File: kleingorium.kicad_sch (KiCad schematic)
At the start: 47 parts, among them J1 4017 Pins, J10 VCC, J11 GND, J12 4046 Comp In, J13 Select, J14 Input, J15 4046 SigIn, J16 4046 Comp, J17 Output, J18 4046 Comp In, J19 4046 Out, J2 4040 Output, J20 4040 Input, J21 4040 Output, J22 4017 Pins, J23 VCC, J24 GND, J25 4017 Fdbk, J26 4017 Fdbk, J3 4040 Input, J4 4046 Out, J5 4046 Comp, J6 Select, J7 Output, J8 Input, J9 4046 SigIn, Q1 2N3904, Q2 2N3904, Q3 2N3904, Q4 2N3904, Q5 2N3904, Q6 2N3904, SW1 4017 Feedback, SW2 4046 CompIn, SW3 Chain, SW4 4017 Feedback, SW5 4046 CompIn

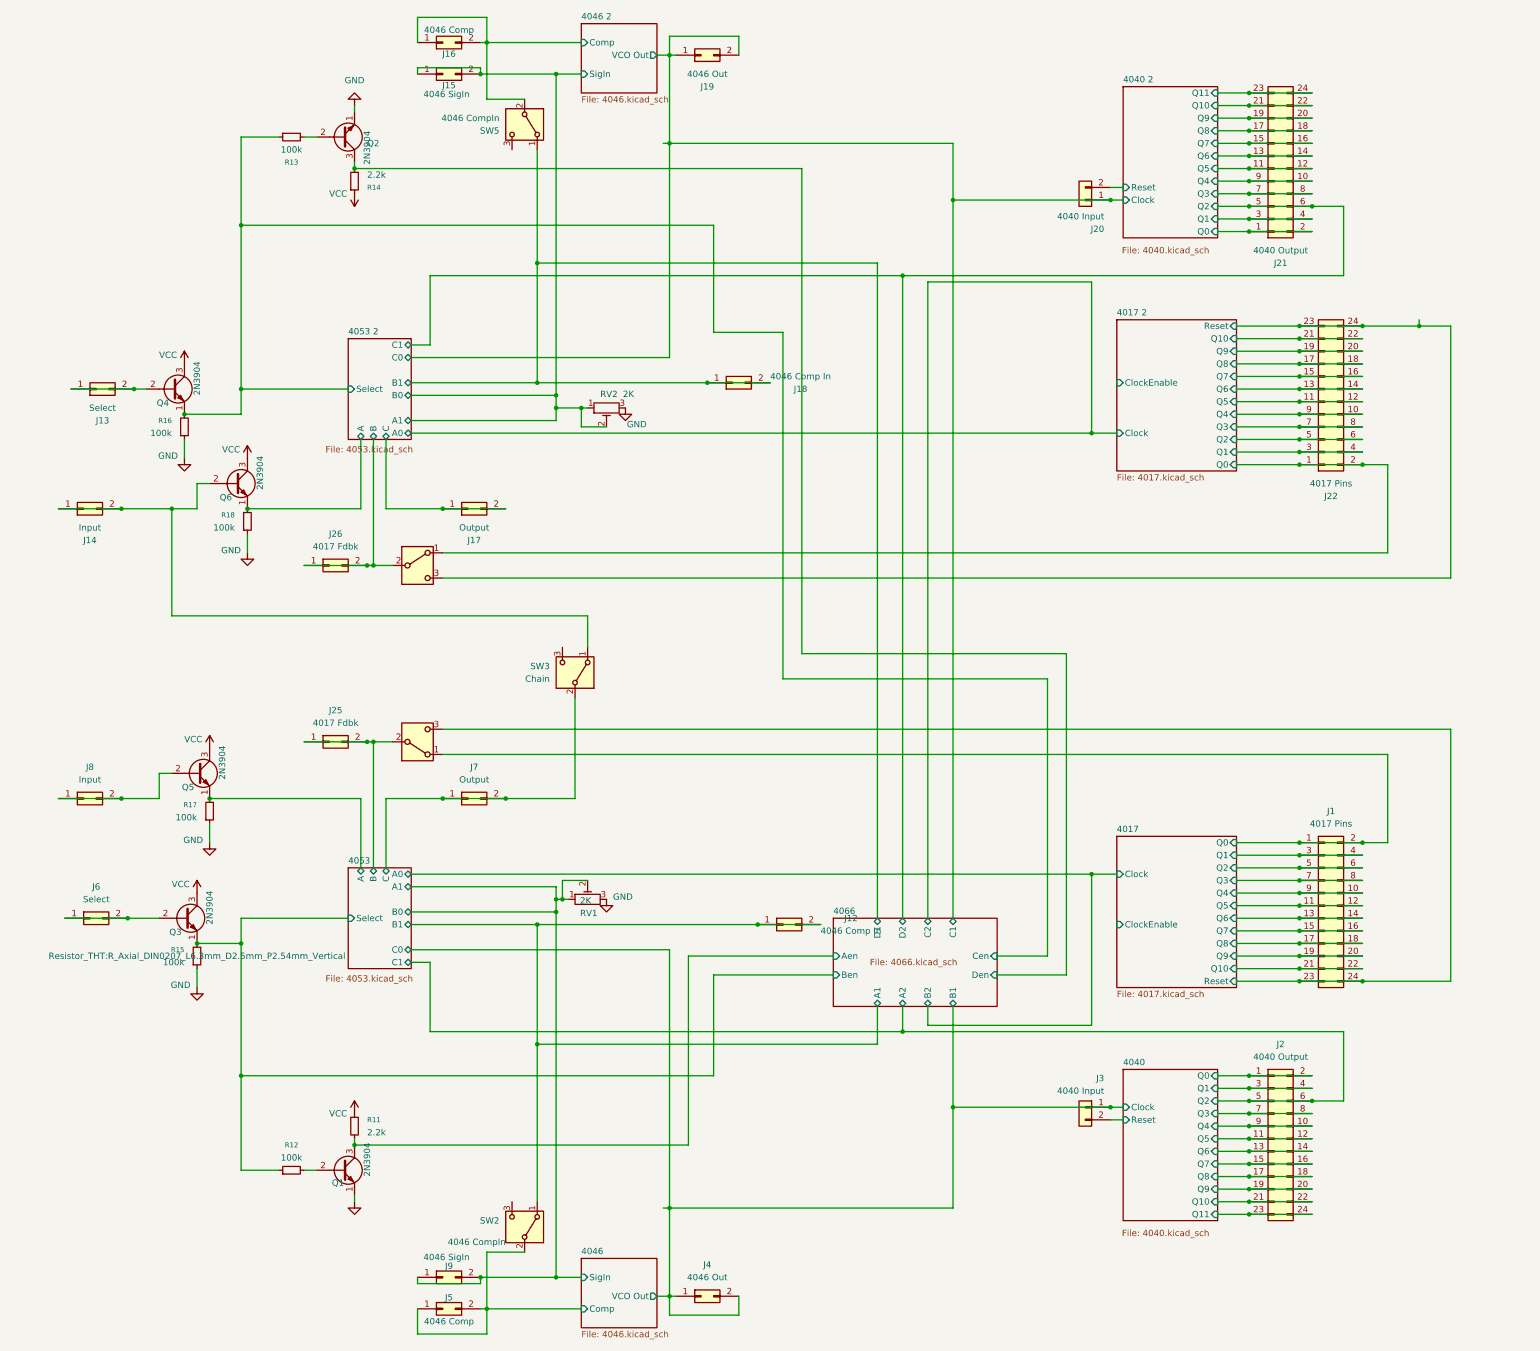
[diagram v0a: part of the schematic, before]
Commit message: v2 initial commit
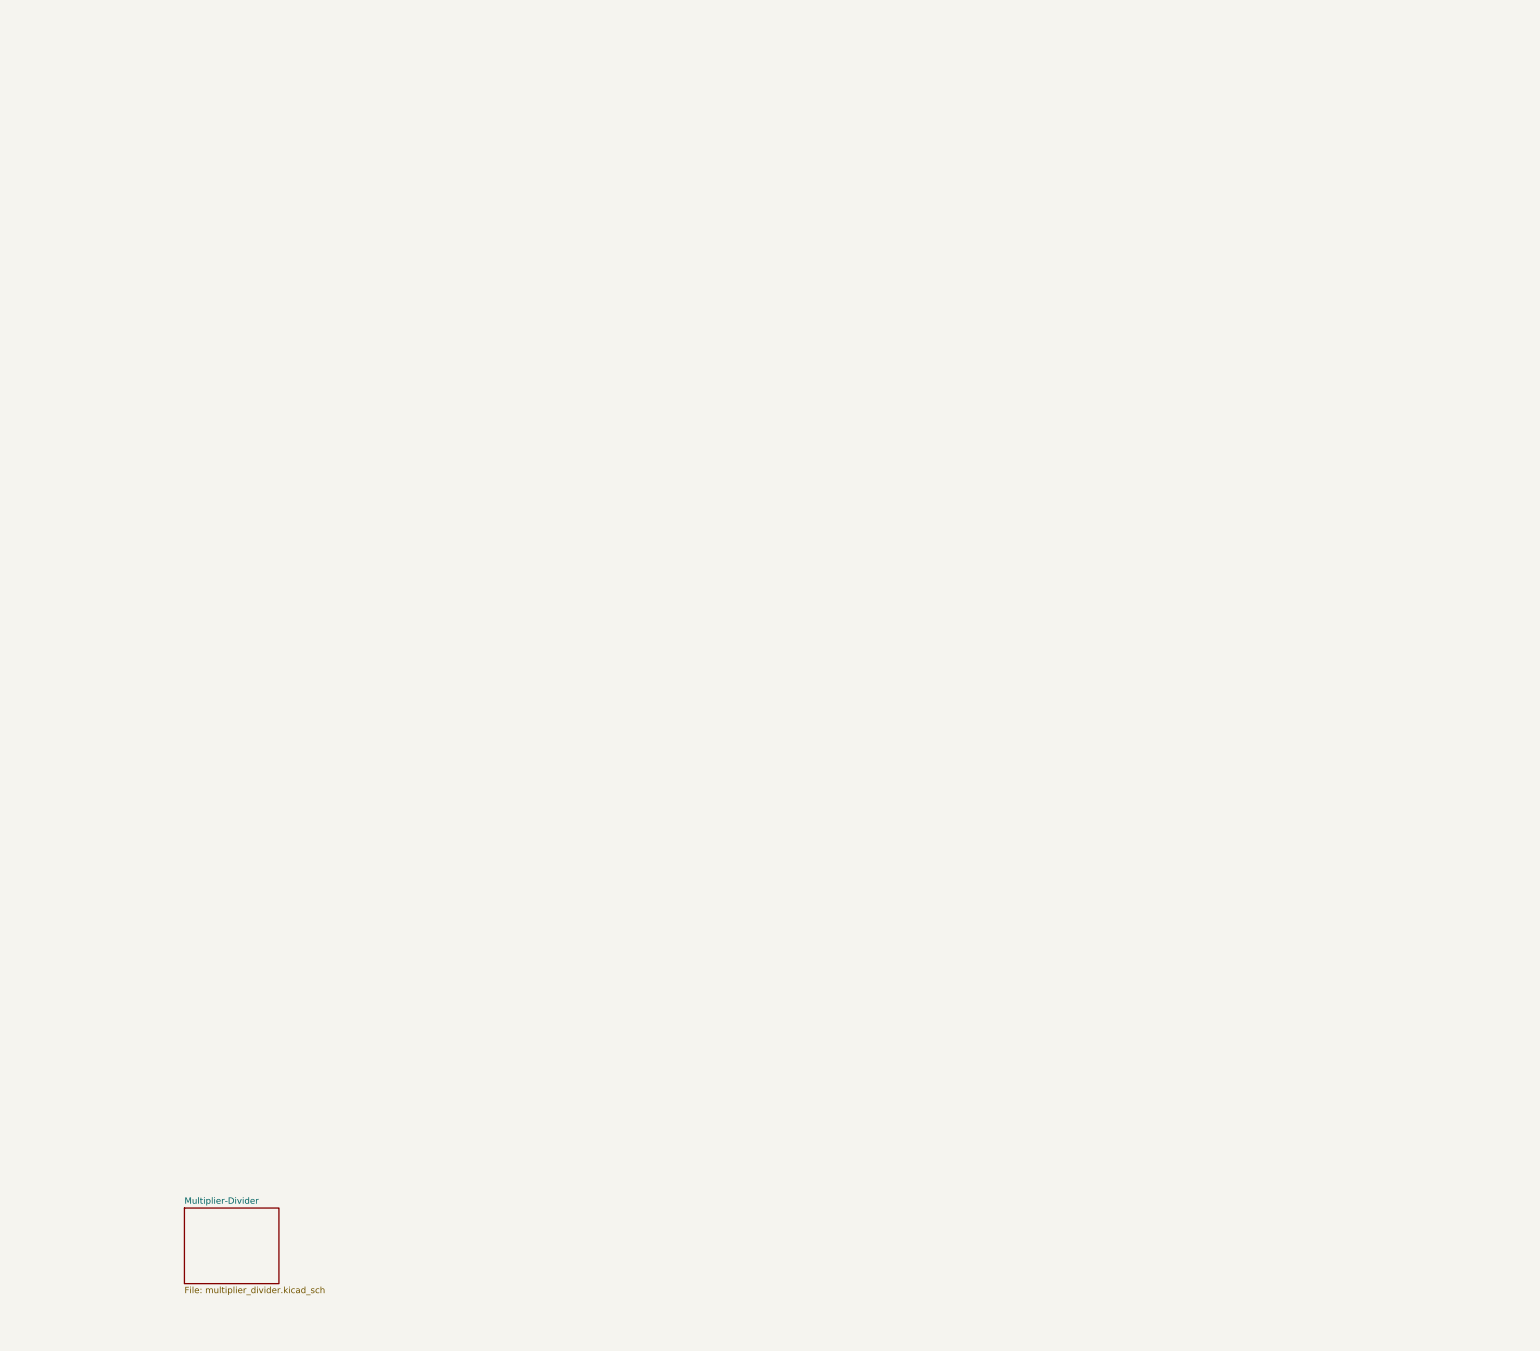
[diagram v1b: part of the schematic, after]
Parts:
- removed J1, J22: 4017 Pins, Connector_PinHeader_2.54mm:PinHeader_2x12_P2.54mm_Vertical, symbol Connector_Generic:Conn_02x12_Odd_Even
- removed J12, J18: 4046 Comp In, Connector_PinHeader_2.54mm:PinHeader_2x01_P2.54mm_Vertical, symbol Connector_Generic:Conn_02x01
- removed J13, J6: Select, Connector_PinHeader_2.54mm:PinHeader_2x01_P2.54mm_Vertical, symbol Connector_Generic:Conn_02x01
- removed J14, J8: Input, Connector_PinHeader_2.54mm:PinHeader_2x01_P2.54mm_Vertical, symbol Connector_Generic:Conn_02x01
- removed J15, J9: 4046 SigIn, Connector_PinHeader_2.54mm:PinHeader_2x01_P2.54mm_Vertical, symbol Connector_Generic:Conn_02x01
- removed J16, J5: 4046 Comp, Connector_PinHeader_2.54mm:PinHeader_2x01_P2.54mm_Vertical, symbol Connector_Generic:Conn_02x01
- removed J17, J7: Output, Connector_PinHeader_2.54mm:PinHeader_2x01_P2.54mm_Vertical, symbol Connector_Generic:Conn_02x01
- removed J19, J4: 4046 Out, Connector_PinHeader_2.54mm:PinHeader_2x01_P2.54mm_Vertical, symbol Connector_Generic:Conn_02x01
- removed J2, J21: 4040 Output, Connector_PinHeader_2.54mm:PinHeader_2x12_P2.54mm_Vertical, symbol Connector_Generic:Conn_02x12_Odd_Even
- removed J20, J3: 4040 Input, Connector_PinHeader_2.54mm:PinHeader_1x02_P2.54mm_Vertical, symbol Connector_Generic:Conn_01x02
- removed J25, J26: 4017 Fdbk, Connector_PinHeader_2.54mm:PinHeader_2x01_P2.54mm_Vertical, symbol Connector_Generic:Conn_02x01
- removed Q1, Q2, Q3, Q4, Q5, Q6: 2N3904, Package_TO_SOT_THT:TO-92_Inline_Wide, symbol Transistor_BJT:2N3904
- removed R11, R14: 2.2k, Resistor_THT:R_Axial_DIN0207_L6.3mm_D2.5mm_P10.16mm_Horizontal, symbol Device:R_Small
- removed R12, R13: 100k, Resistor_THT:R_Axial_DIN0207_L6.3mm_D2.5mm_P10.16mm_Horizontal, symbol Device:R_Small
- removed R15, R16, R17, R18: 100k, Resistor_THT:R_Axial_DIN0207_L6.3mm_D2.5mm_P2.54mm_Vertical, symbol Device:R_Small
- removed RV1, RV2: 2K, Potentiometer_THT:Potentiometer_Bourns_3296W_Vertical, symbol Device:R_Potentiometer_Trim
- removed SW1, SW4: 4017 Feedback, Button_Switch_THT:SW_CK_JS202011CQN_DPDT_Straight, symbol Switch:SW_DPDT_x2
- removed SW2, SW5: 4046 CompIn, Button_Switch_THT:SW_E-Switch_EG1271_SPDT, symbol Switch:SW_SPDT
- removed SW3: Chain, Button_Switch_THT:SW_E-Switch_EG1271_SPDT, symbol Switch:SW_SPDT
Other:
- removed sheet 4017
- removed sheet 4017 2
- removed sheet 4040
- removed sheet 4040 2
- removed sheet 4046
- removed sheet 4046 2
- removed sheet 4053
- removed sheet 4053 2
- removed sheet 4066
- added sheet Multiplier-Divider (multiplier_divider.kicad_sch)
